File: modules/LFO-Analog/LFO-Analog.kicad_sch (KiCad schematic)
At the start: 56 parts, among them Q1 2N3904, Q2 2N3904, Q3 2N3904, Q4 2N3904, U1 TL074, U2 TL074

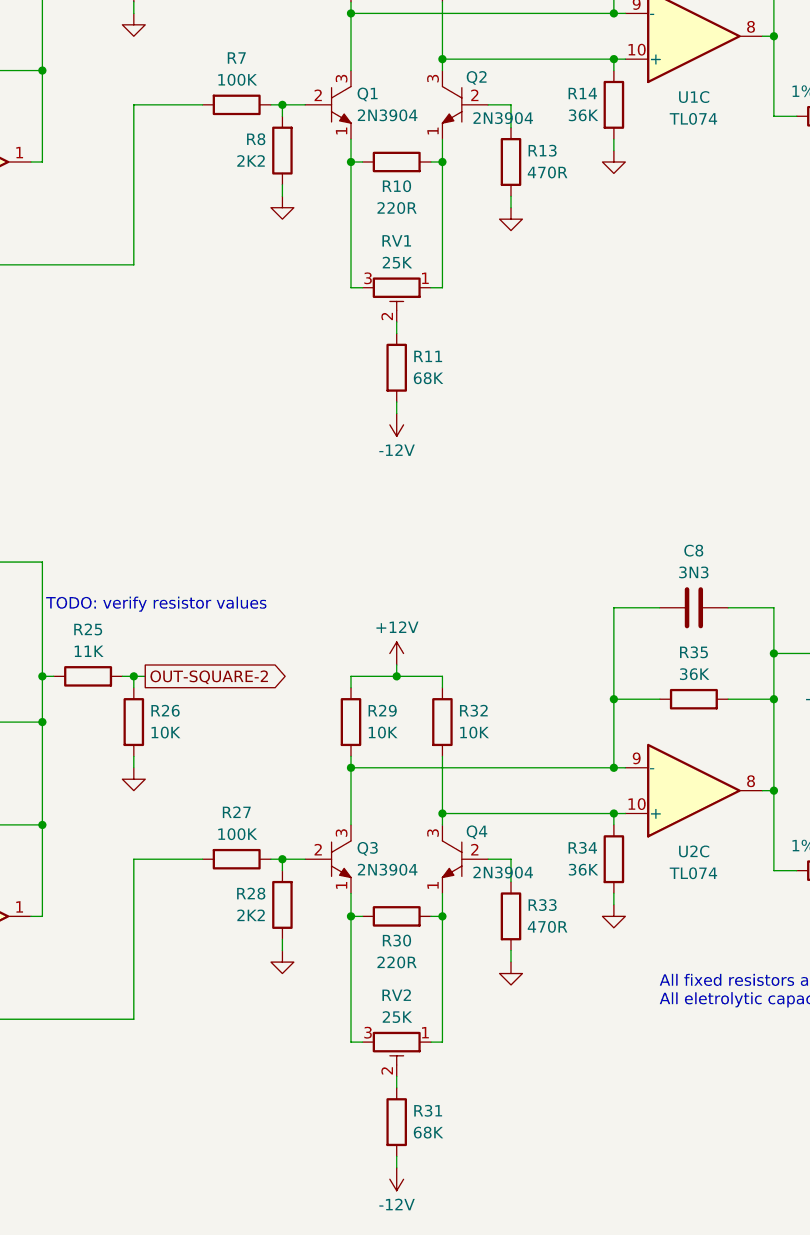
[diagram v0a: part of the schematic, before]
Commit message: LFO-Analog: BOM testing - update some fields
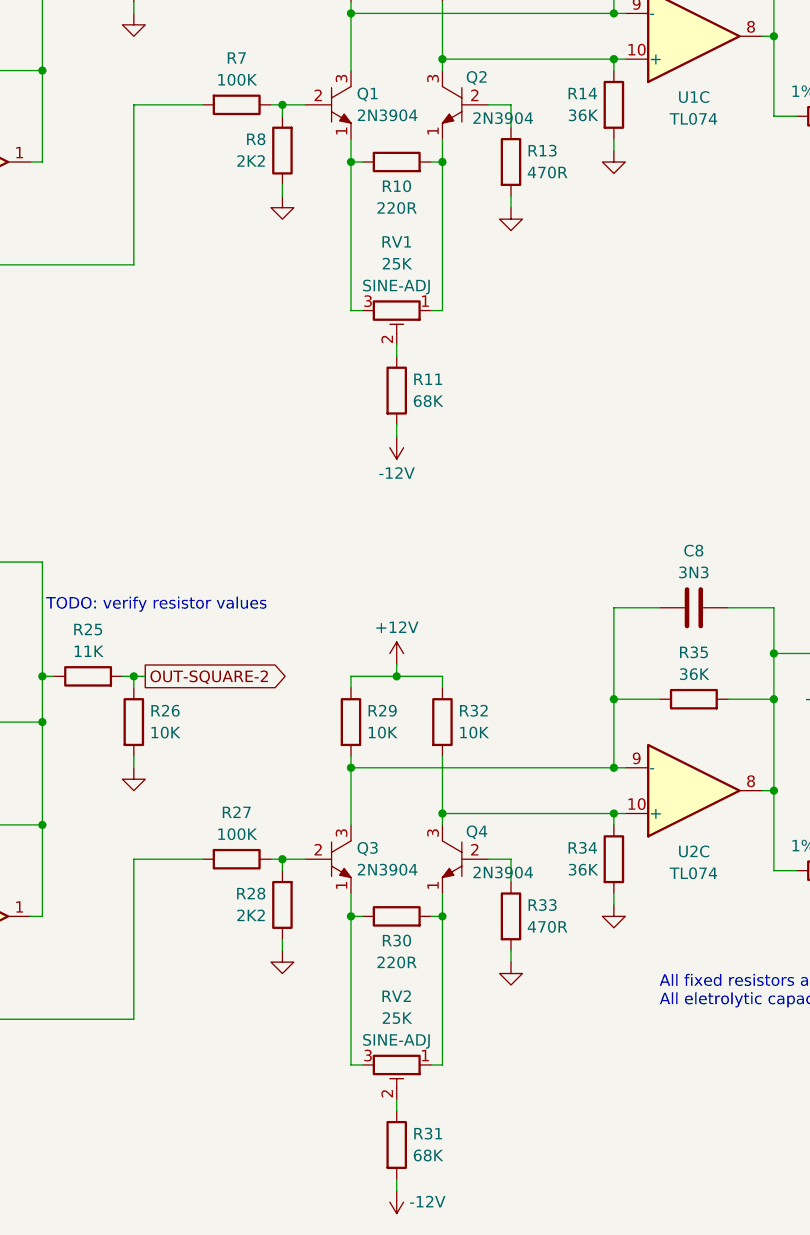
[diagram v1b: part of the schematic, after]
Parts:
- RV1, RV2: Label [label] -> SINE-ADJ
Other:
- moved on the sheet: R11, R31, RV1, RV2
